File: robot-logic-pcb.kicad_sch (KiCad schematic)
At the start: 26 parts, among them U1 NRF24L01_Breakout, U2 XIAO-ESP32-S3-DIP

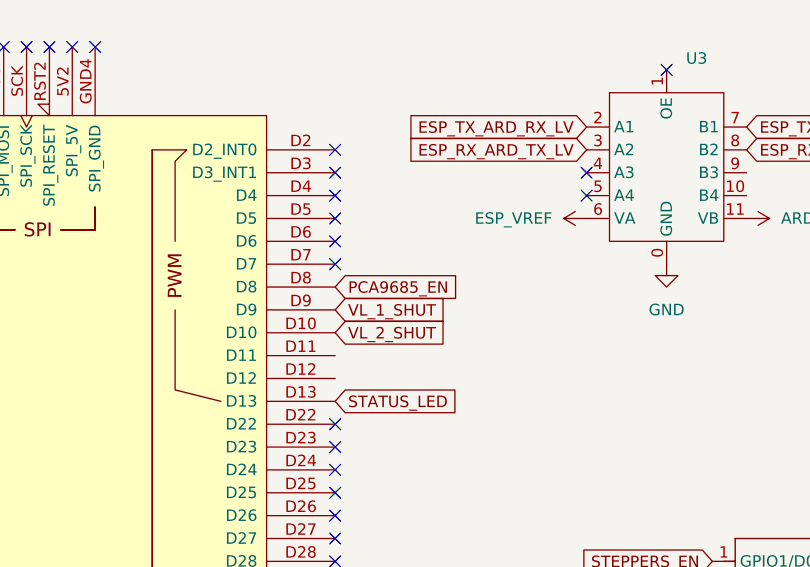
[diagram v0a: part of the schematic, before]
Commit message: forgot to save sch lol
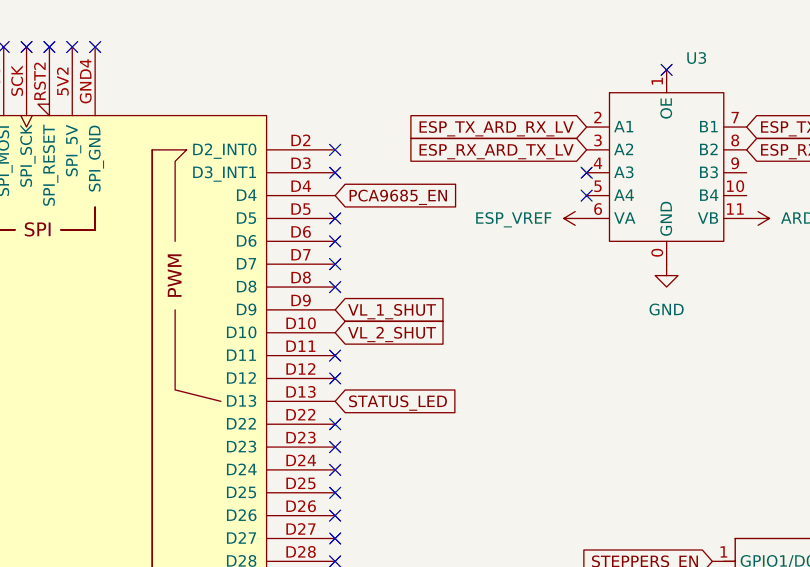
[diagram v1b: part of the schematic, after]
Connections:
- net PCA9685_EN: now also A1.D4; no longer A1.D8
- no-connect marks 78 -> 80
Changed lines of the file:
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@@
+	)
+	(no_connect
+		(at 99.06 90.17)
 	)
 	(no_connect
@@
 	)
 	(no_connect
+		(at 99.06 97.79)
+	)
+	(no_connect
 		(at 33.02 166.37)
 	)
@@
 	)
 	(no_connect
-		(at 99.06 80.01)
-	)
-	(no_connect
 		(at 62.23 63.5)
 	)
@@
 	(no_connect
 		(at 72.39 63.5)
+	)
+	(no_connect
+		(at 99.06 100.33)
 	)
 	(no_connect
@@
 		)
 	)
+	(global_label "PCA9685_EN"
+		(shape input)
+		(at 99.06 80.01 0)
+		(fields_autoplaced yes)
+		(effects
+			(font
+				(size 1.27 1.27)
+			)
+			(justify left)
+		)
+		(property "Intersheetrefs" "${INTERSHEET_REFS}"
+			(at 113.9589 80.01 0)
+			(effects
+				(font
+					(size 1.27 1.27)
+				)
+				(justify left)
+				(hide yes)
+			)
+		)
+	)
 	(global_label "SC_STEP"
 		(shape input)
@@
 				(hide yes)
 			)
-		)
-	)
-	(global_label "PCA9685_EN"
-		(shape input)
-		(at 99.06 90.17 0)
-		(fields_autoplaced yes)
-		(effects
-			(font
-				(size 1.27 1.27)
-			)
-			(justify left)
-		)
-		(property "Intersheetrefs" "${INTERSHEET_REFS}"
-			(at 113.9589 90.17 0)
-			(effects
-				(font
-					(size 1.27 1.27)
-				)
-				(justify left)
-				(hide yes)
-			)
